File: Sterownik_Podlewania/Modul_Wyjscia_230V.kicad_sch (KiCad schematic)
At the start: 10 parts, among them J6 Screw_Terminal_01x02, K1 SANYOU_SRD_Form_C, Q1 BC547, SW1 SW_Nidec_CAS-120A1

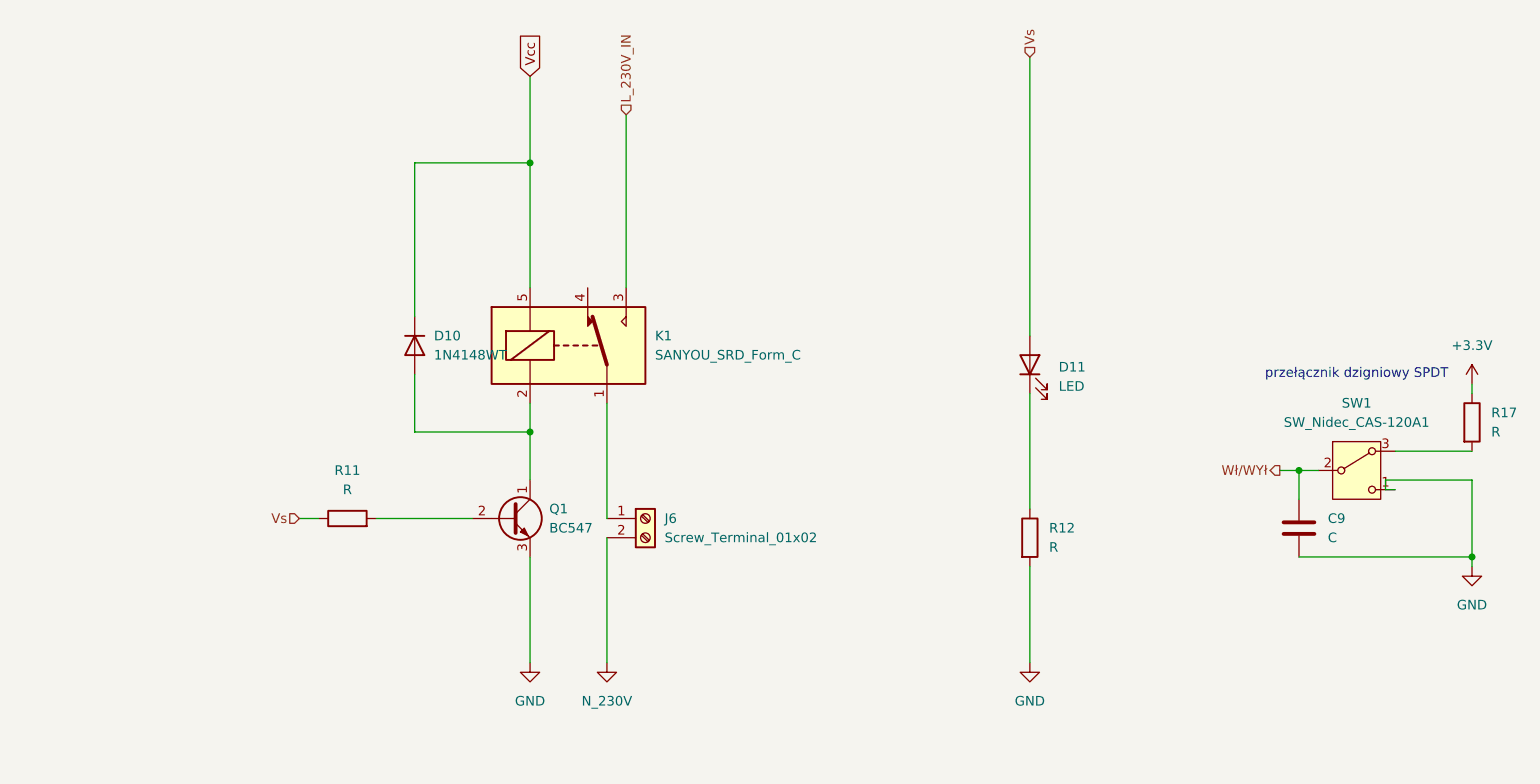
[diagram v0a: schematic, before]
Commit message: Poprawki estetyczne schematu
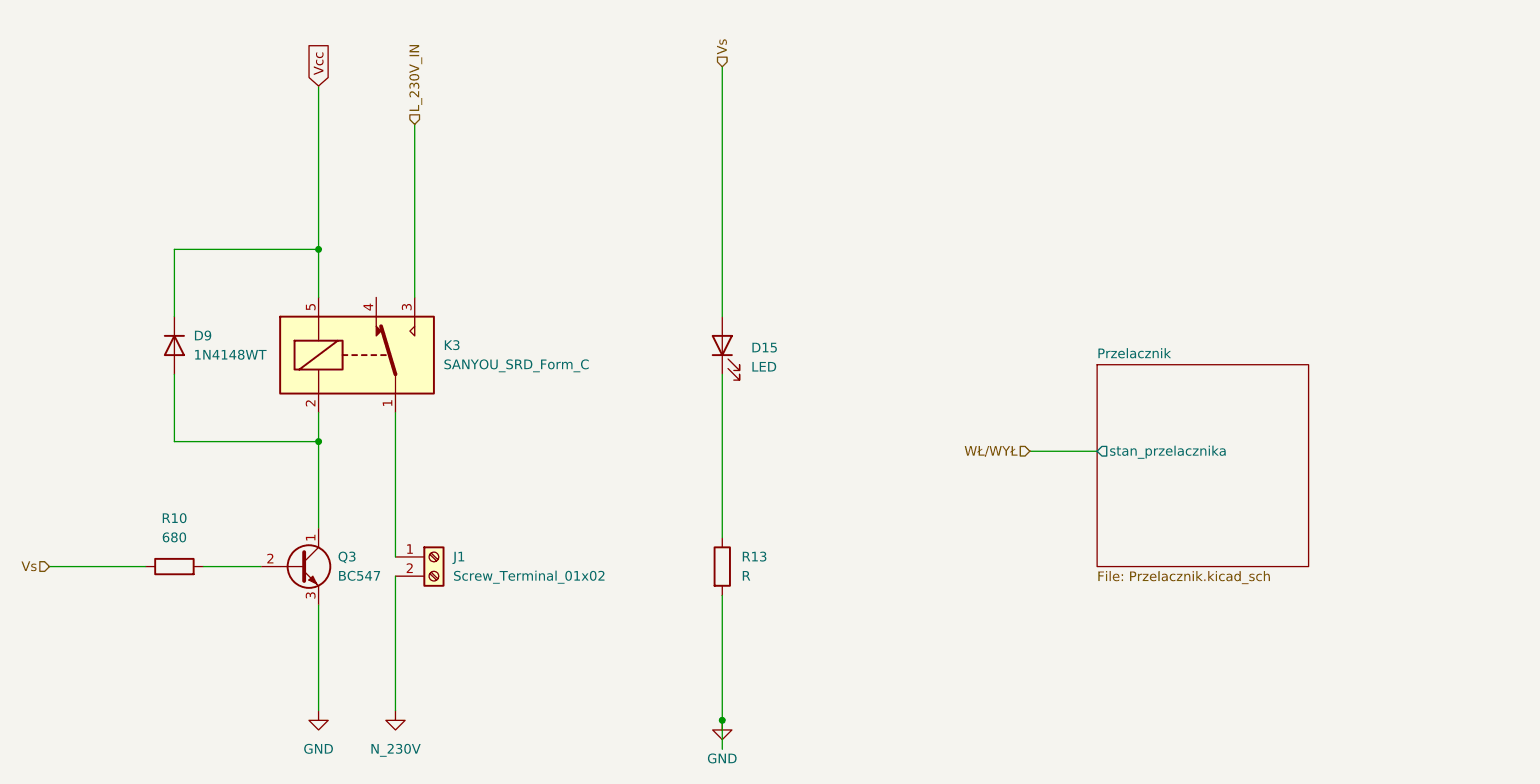
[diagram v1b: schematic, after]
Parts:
- removed C9: C, symbol Device:C
- removed D10: 1N4148WT, Diode_SMD:D_SOD-523, symbol Diode:1N4148WT
- removed D11: LED, LED_SMD:LED_1206_3216Metric, symbol Device:LED
- removed J6: Screw_Terminal_01x02, TerminalBlock:TerminalBlock_Wuerth_691311400102_P7.62mm, symbol Connector:Screw_Terminal_01x02
- removed K1: SANYOU_SRD_Form_C, Relay_THT:Relay_SPDT_SANYOU_SRD_Series_Form_C, symbol Relay:SANYOU_SRD_Form_C
- removed Q1: BC547, Package_TO_SOT_THT:TO-92_Inline, symbol Transistor_BJT:BC547
- removed R11, R12, R17: R, Resistor_SMD:R_1206_3216Metric, symbol Device:R
- removed SW1: SW_Nidec_CAS-120A1, Button_Switch_SMD:Nidec_Copal_CAS-120A, symbol Switch:SW_Nidec_CAS-120A1
- added D15: LED, LED_SMD:LED_1206_3216Metric, symbol Device:LED
- added D9: 1N4148WT, Diode_SMD:D_SOD-523, symbol Diode:1N4148WT
- added J1: Screw_Terminal_01x02, TerminalBlock:TerminalBlock_MaiXu_MX126-5.0-02P_1x02_P5.00mm, symbol Connector:Screw_Terminal_01x02
- added K3: SANYOU_SRD_Form_C, Relay_THT:Relay_SPDT_SANYOU_SRD_Series_Form_C, symbol Relay:SANYOU_SRD_Form_C
- added Q3: BC547, Package_TO_SOT_THT:TO-92_Inline, symbol Transistor_BJT:BC547
- added R10: 680, Resistor_SMD:R_1206_3216Metric, symbol Device:R
- added R13: R, Resistor_SMD:R_1206_3216Metric, symbol Device:R
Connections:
- net GND: now also Q3.3 (E), R13.2
- net L_230V_IN: now also K3.3
- net N_230V: now also J1.2 (Pin_2)
- net Vcc: now also D9.1 (K), K3.5
- net Vs: now also D15.2 (A), R10.1
- new net: D9.2 (A), K3.2, Q3.1 (C)
- new net: Q3.2 (B), R10.2
- new net: D15.1 (K), R13.1
- new net: J1.1 (Pin_1), K3.1
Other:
- added sheet Przelacznik (Przelacznik.kicad_sch)
- note removed: "przełącznik dzigniowy SPDT"
